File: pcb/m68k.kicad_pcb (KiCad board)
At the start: 2 copper layers, 100 x 100 mm, 120 parts, among them J1 USB_B_Micro, J2 Mini-DIN-6, J4 DB15_Male_HighDensity, J8 Micro_SD_Card, U1 93LC56, U10 25LCxxx, U11 TXB0108DQSR, U12 TXB0108DQSR, U13 iCE40-HX4K-TQ144, U14 ADV7125KSTZ50, U15 74LVC1G17, U16 LD1117S33TR_SOT223, U17 LD1117S12TR_SOT223, U18 ATL431BQDBZR, U2 68000D, U3 FT2232H, U4 TXB0108DQSR, U5 TXB0108DQSR, U6 TXB0108DQSR, U7 SN74LVC8T245PWR, U8 SN74LVC8T245PWR, U9 AS6C1616, X1 ASV-12.000MHz

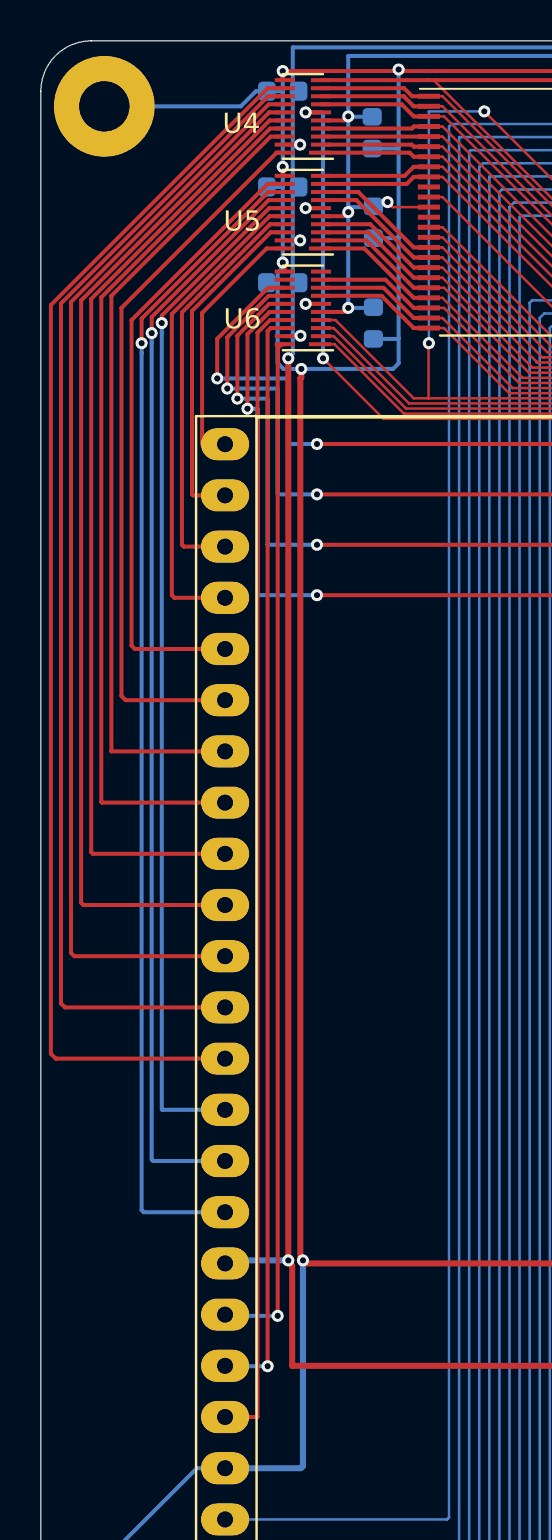
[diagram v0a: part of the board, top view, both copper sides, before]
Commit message: Finished
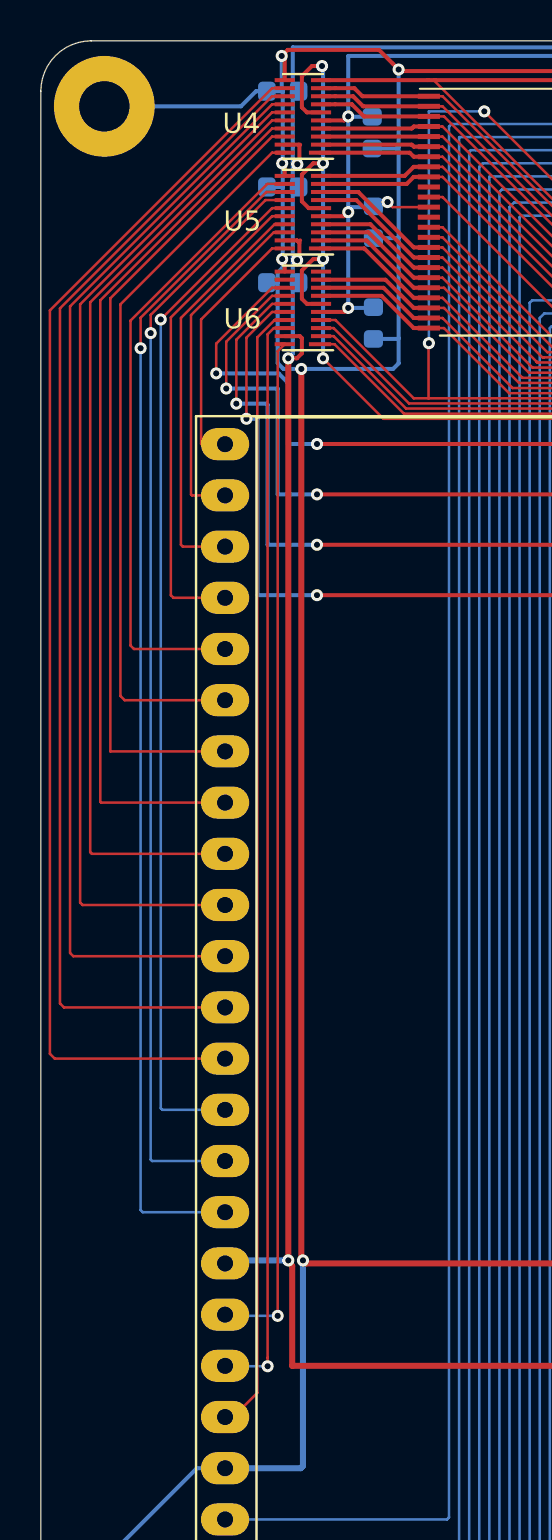
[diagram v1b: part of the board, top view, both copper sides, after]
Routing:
- net ADDR_OE: track 78.3 -> 87.1 mm
- net GND: track 773.9 -> 776.4 mm
- net +5V: track 346.0 -> 348.3 mm, vias 14 -> 13
- net /A23: track 57.0 -> 56.2 mm
- net /A10: track 35.8 -> 36.4 mm
